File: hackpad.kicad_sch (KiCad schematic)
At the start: 40 parts, among them J1 OLED_Display, SW1 SW_Push, SW10 SW_Push, SW11 SW_Push, SW12 SW_Push, SW13 SW_Push, SW14 SW_Push, SW15 SW_Push, SW16 SW_Push, SW17 SW_Push, SW18 SW_Push, SW19 SW_Push, SW2 SW_Push, SW3 SW_Push, SW4 SW_Push, SW5 SW_Push, SW6 SW_Push, SW7 SW_Push, SW8 SW_Push, SW9 SW_Push, U1 SEEED-XIAO

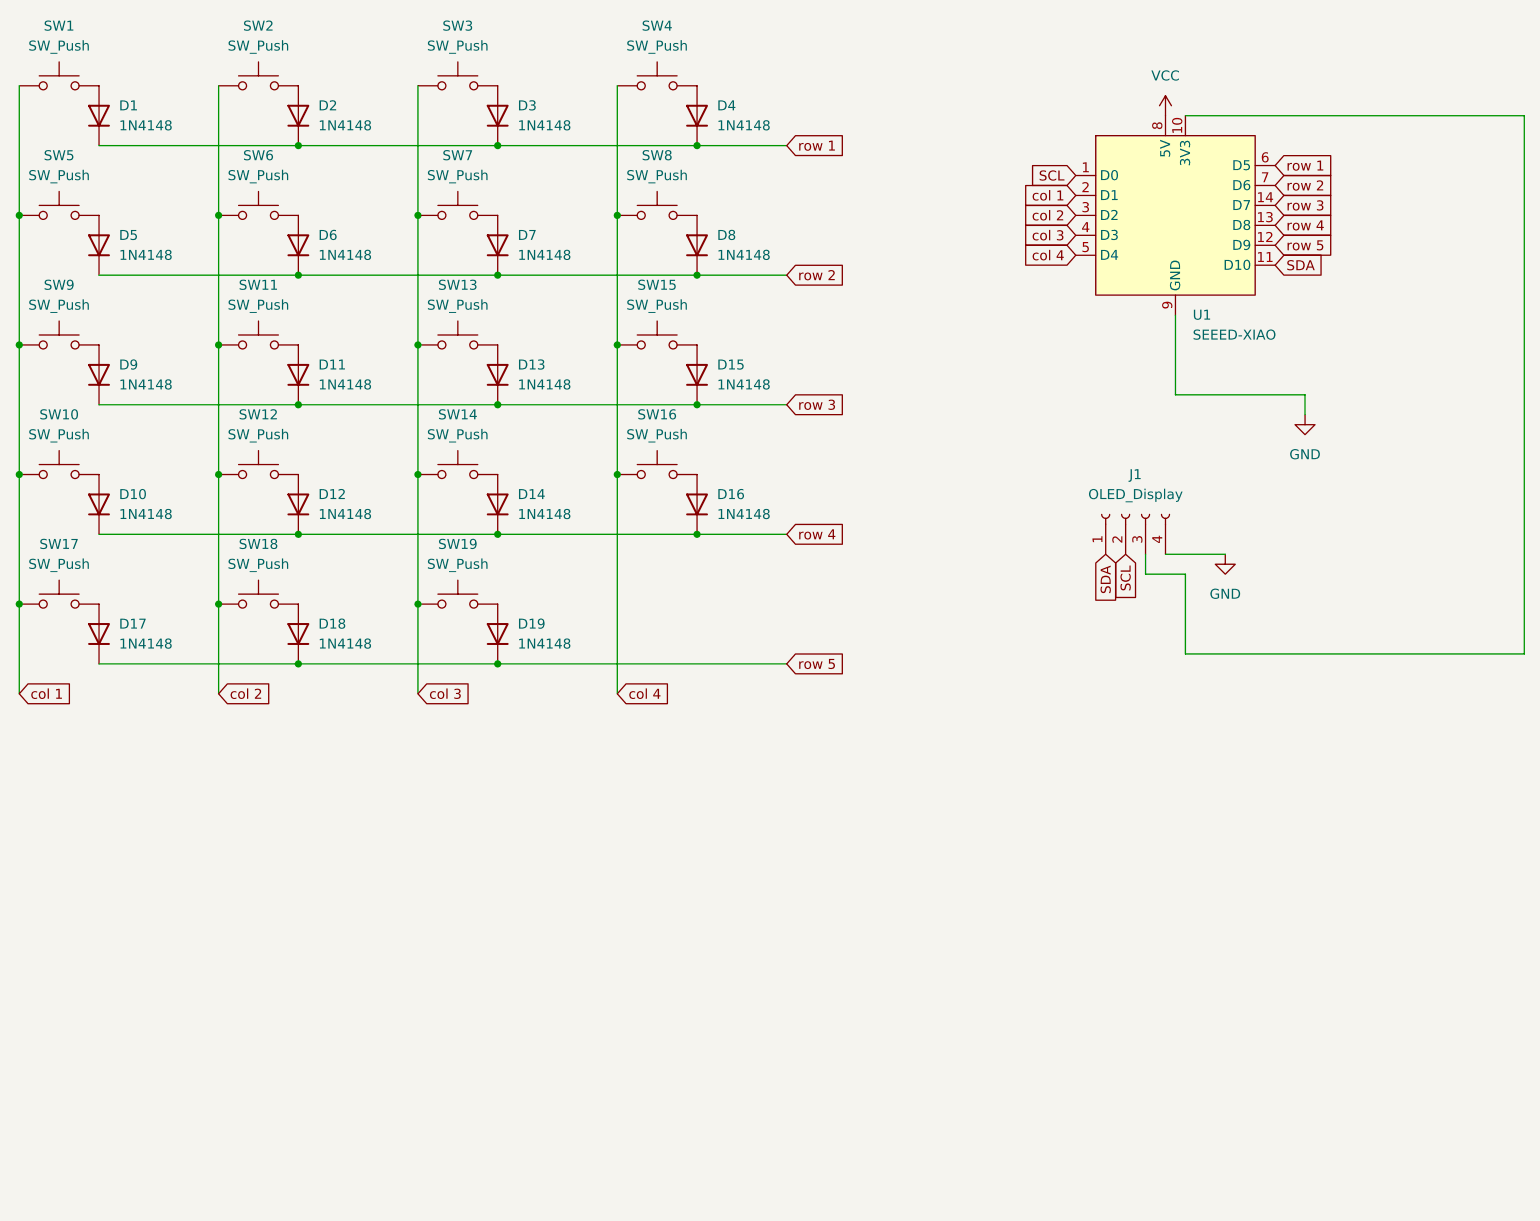
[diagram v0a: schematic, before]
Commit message: idk
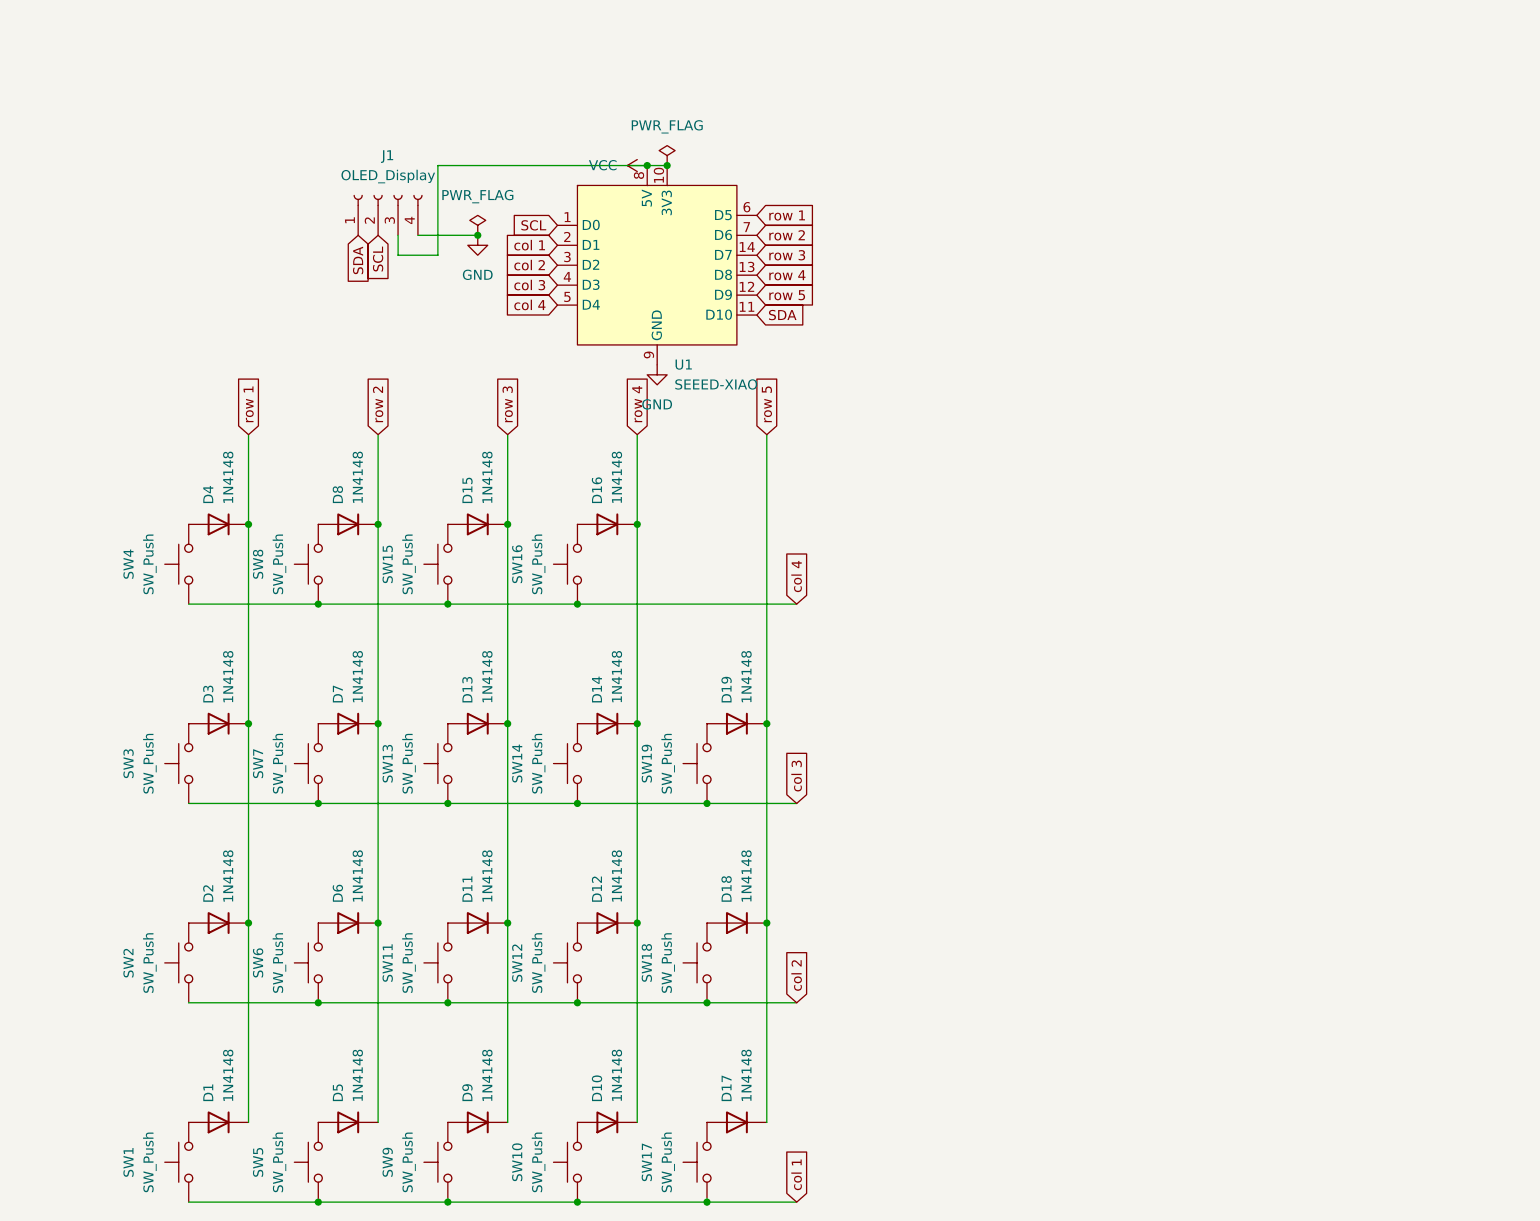
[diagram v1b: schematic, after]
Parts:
- J1: footprint (none) -> e:SSD1306-0.91-OLED-4pin-128x32
- SW1, SW10, SW11, SW12, SW13, SW14, SW15, SW16, SW17, SW18, SW19, SW2, SW3, SW4, SW5, SW6, SW7, SW8, SW9: footprint (none) -> Button_Switch_Keyboard:SW_Cherry_MX_1.00u_PCB
- U1: footprint XIAO_PCB:XIAO-14P-SMD-2.54-21x17.8MM -> Seeeduino-xiao-rp2040-KiCAD-Library:MOUDLE14P-2.54-21X17.8MM
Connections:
- net VCC: now also J1.3 (Pin_3), U1.10 (3V3)
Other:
- moved on the sheet: D1, D10, D11, D12, D13, D14, D15, D16, D17, D18, D19, D2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
